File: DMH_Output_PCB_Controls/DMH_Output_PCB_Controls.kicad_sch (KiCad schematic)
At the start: 14 parts, among them J1 TRS_Jack_6.35mm_Sw, J2 TRS_Jack_6.35mm_Sw, J200 IDC_02x05, J21 Conn_01x02, J22 Conn_01x02, J24 Conn_01x02, J25 Conn_01x02, J3 TRS_Jack_6.35mm_Sw, J4 TRS_Jack_6.35mm_Sw, J5 TRS_Jack_6.35mm_Sw, J6 TRS_Jack_6.35mm_Sw, J7 TRS_Jack_6.35mm_Sw, J8 TRS_Jack_6.35mm_Sw, J9 TRS_Jack_6.35mm_Sw

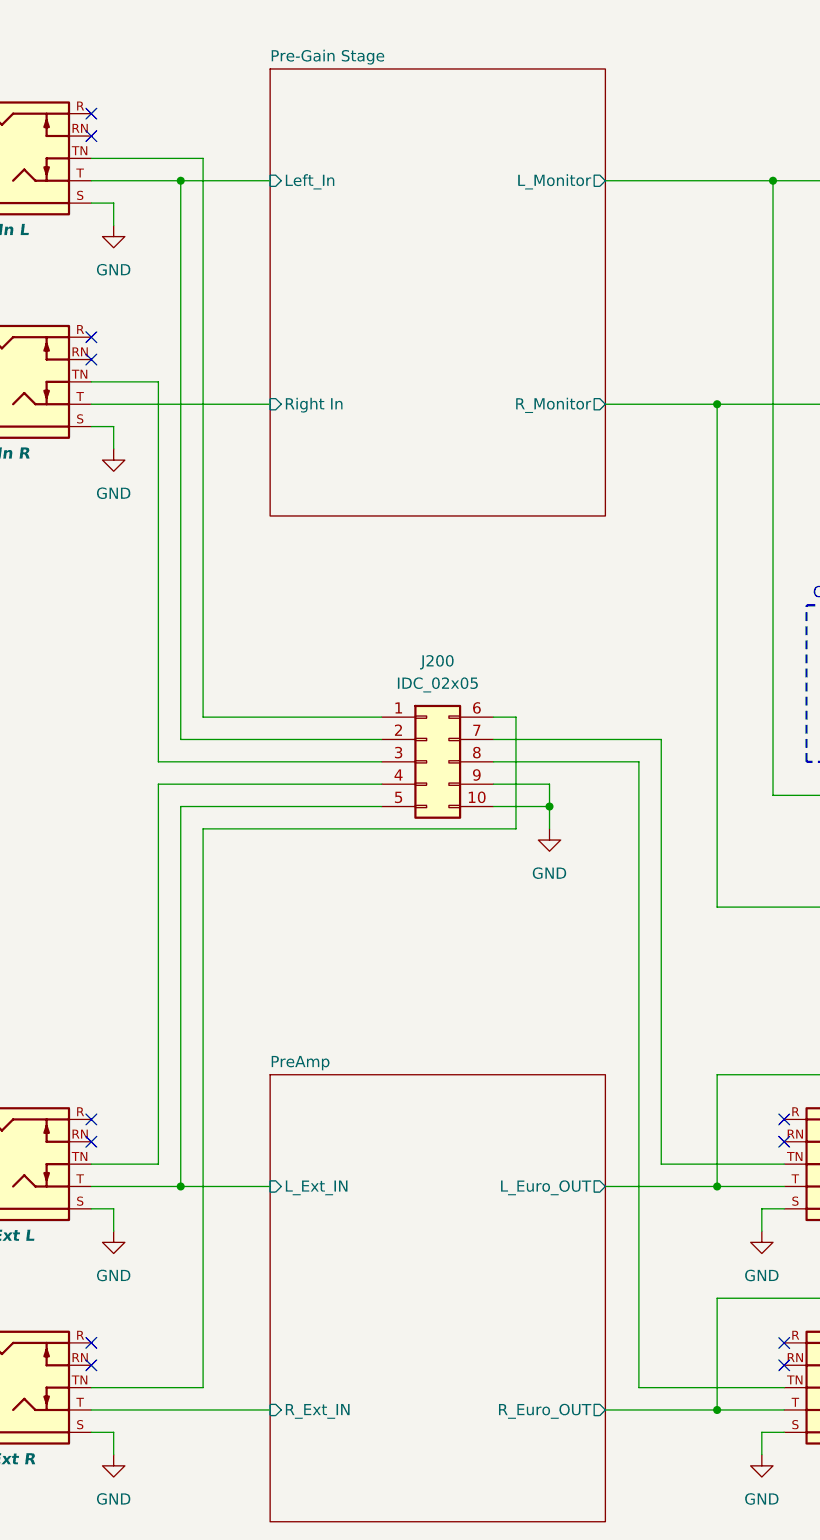
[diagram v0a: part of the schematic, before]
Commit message: Prep for Main and MZ PCBs design in progress
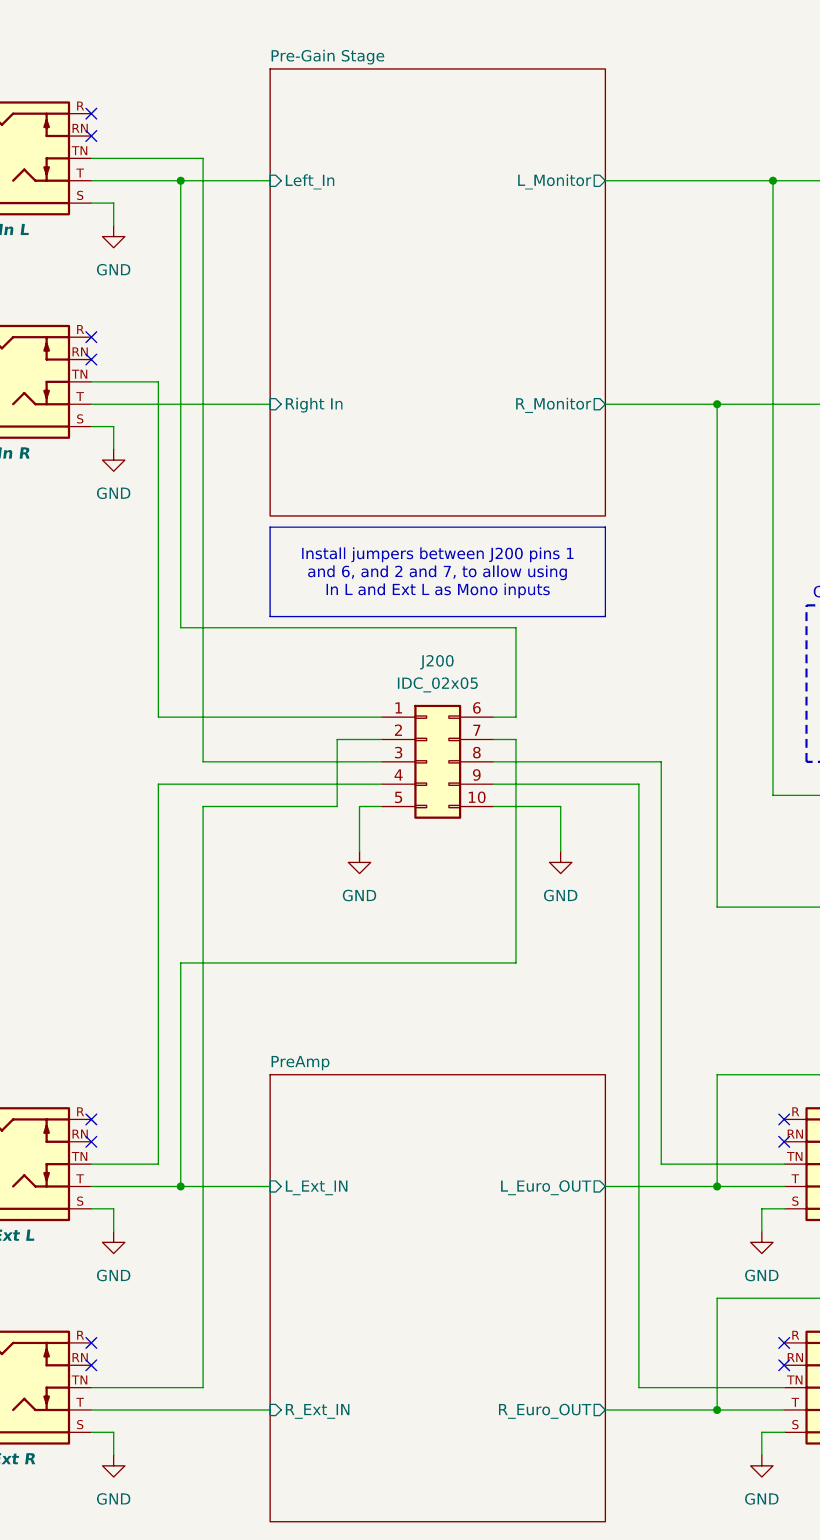
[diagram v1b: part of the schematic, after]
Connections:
- net GND: now also J200.5 (Pin_5); no longer J200.9 (Pin_9)
- net Pre-Gain Stage/Left_In: now also J200.6 (Pin_6); no longer J200.2 (Pin_2)
- net PreAmp/L_Ext_IN: now also J200.7 (Pin_7); no longer J200.5 (Pin_5)
- net at J7.TN (2): now also J200.2 (Pin_2); no longer J200.6 (Pin_6)
- net at J2.TN (2): now also J200.1 (Pin_1); no longer J200.3 (Pin_3)
- net at J9.TN (2): now also J200.9 (Pin_9); no longer J200.8 (Pin_8)
- net at J1.TN (2): now also J200.3 (Pin_3); no longer J200.1 (Pin_1)
- net at J8.TN (2): now also J200.8 (Pin_8); no longer J200.7 (Pin_7)
